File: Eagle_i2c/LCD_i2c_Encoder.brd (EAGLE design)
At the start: 100 x 99 mm, 8 parts, among them J1 455-1750-1-ND, U1 ARDUINOR3-BPLACE

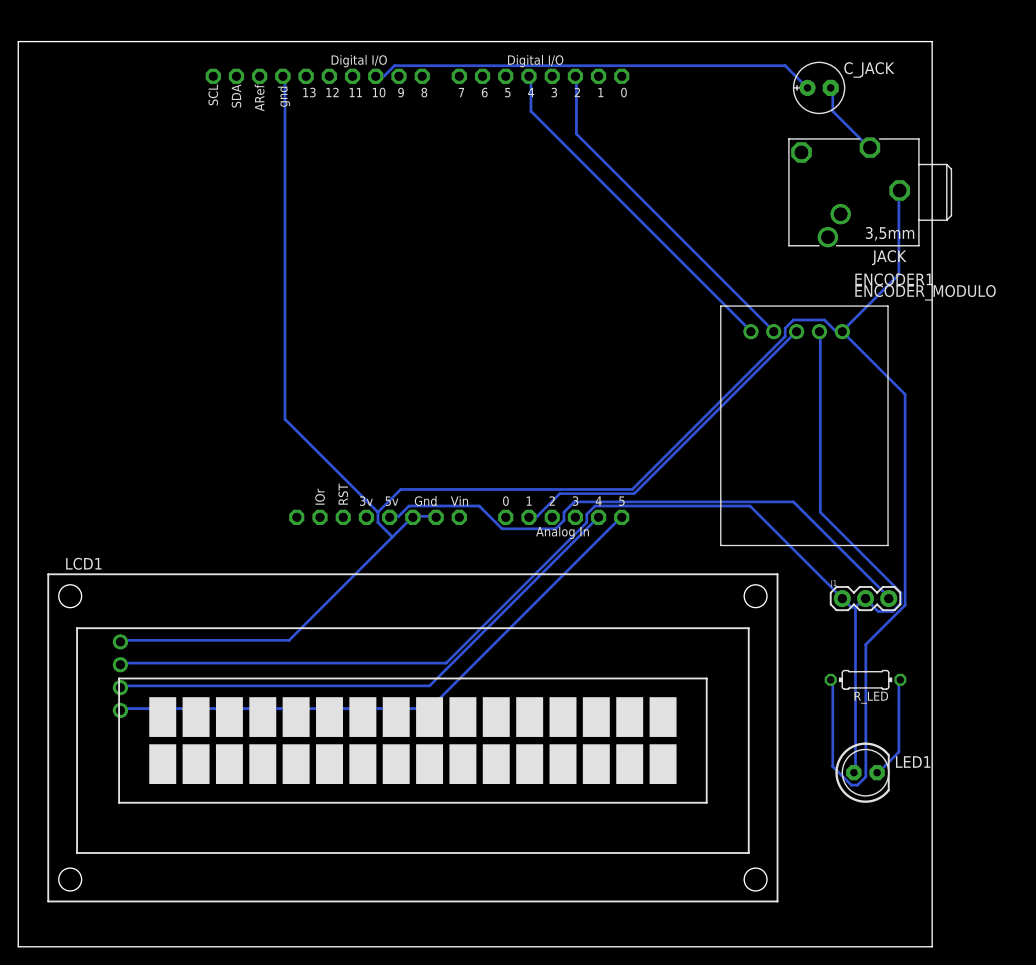
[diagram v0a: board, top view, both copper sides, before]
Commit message: Version final circuito Chladni
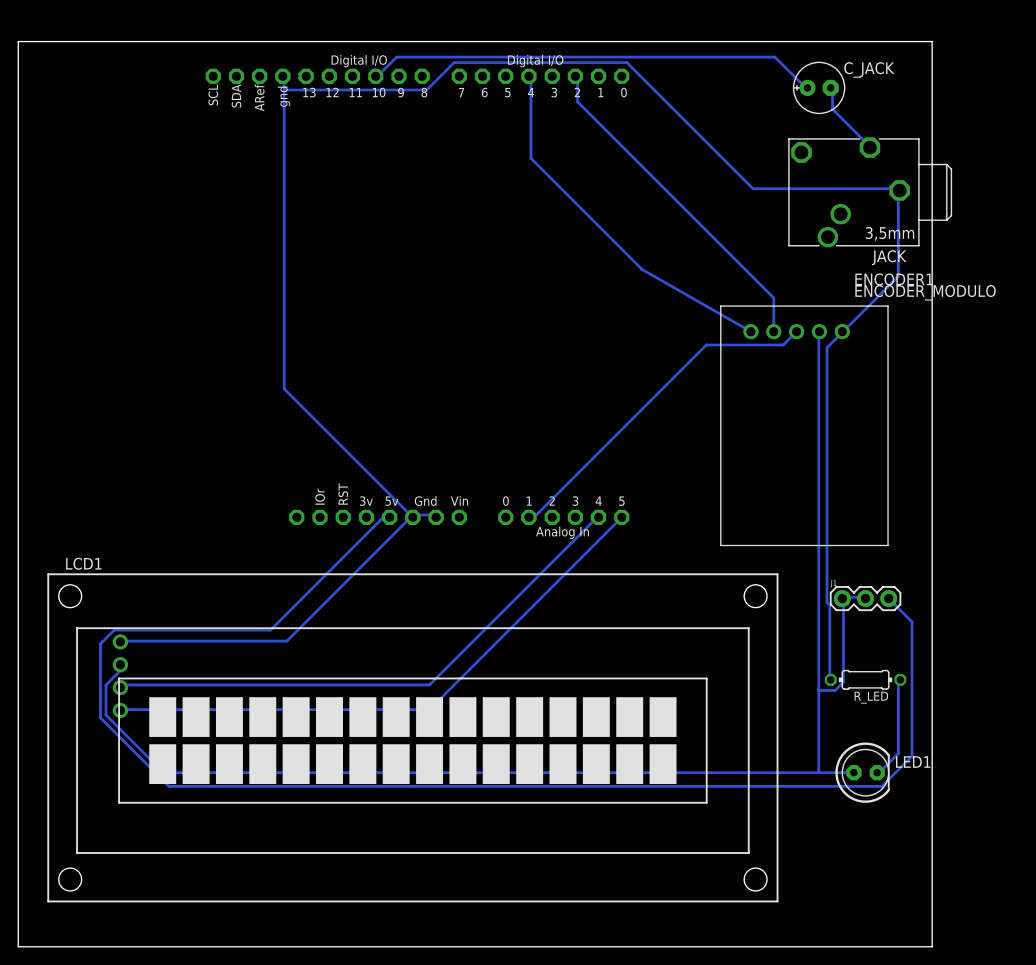
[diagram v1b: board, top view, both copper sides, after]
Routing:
- net N$5: track 62.4 -> 157.0 mm
- net GND: track 242.1 -> 226.3 mm
- net VCC: track 150.8 -> 153.9 mm
- net N$17: track 38.0 -> 40.1 mm
- net N$1: track 48.7 -> 49.5 mm

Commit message: Version para imprimir ICAT, Gerbers incluidos
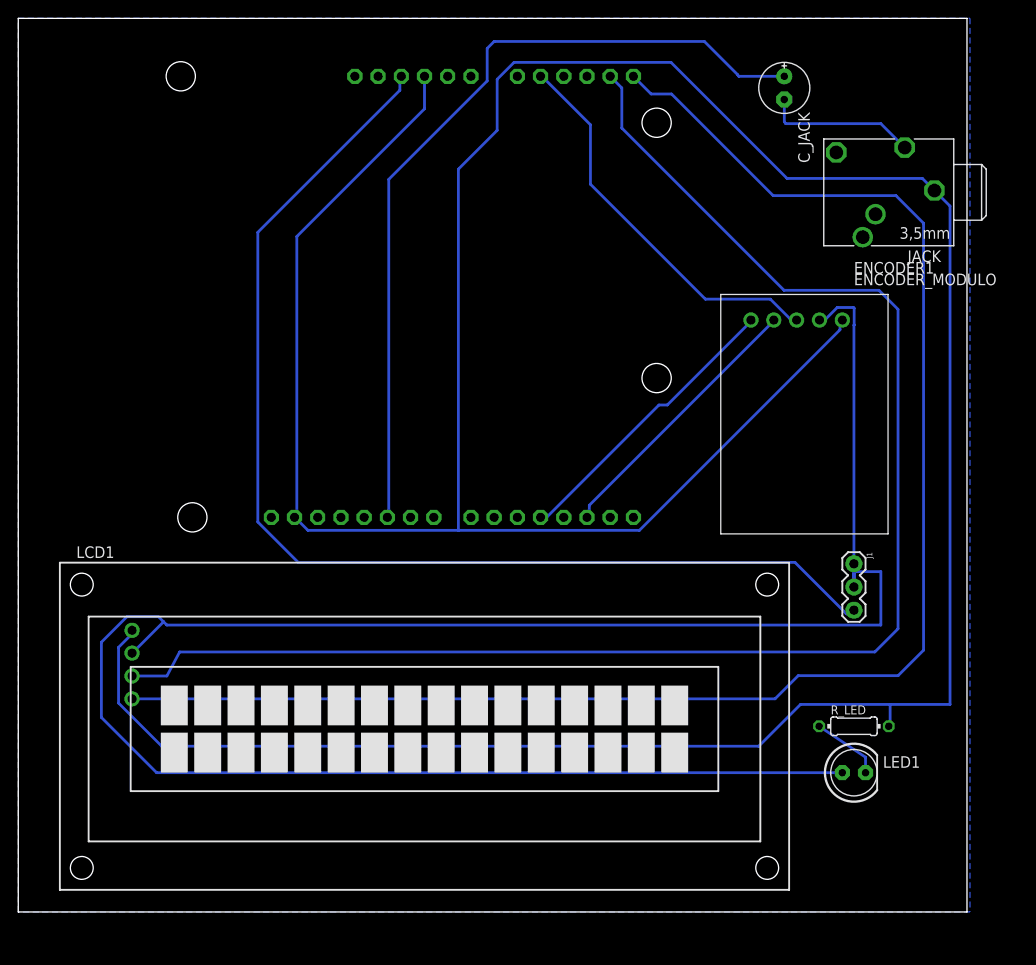
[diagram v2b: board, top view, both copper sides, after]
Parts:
- removed U1: ARDUINOR3-BPLACE, adafruit:ARDUINOR3-BPLACE
- added U$1: ARDUINOUNO, Arduino_Espejo:ARDUINO
- moved R_LED 5.24 mm to (91.4, 5.08), turned to 0 degrees
- moved J1 4.02 mm to (91.4, 22.9), turned to 270 degrees
- moved C_JACK 3.81 mm to (83.8, 74.9), turned to 270 degrees
- moved JACK 3.81 mm to (95.2, 63.5)
- moved LCD1 1.80 mm to (44.5, 5.08)
- moved ENCODER1 1.27 mm to (90.2, 49.5)
- moved LED1 1.27 mm to (91.4, 0.00)
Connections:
- new net GND1: U$1.GND1
- net 3V: now also U$1.3V; no longer U1.3V
- net GND: now also U$1.GND, U$1.GND2; no longer U1.GND, U1.GND1, U1.GND2
- net N$1: now also U$1.D10; no longer U1.D10
- net N$17: now also U$1.D4; no longer U1.D4
- net N$18: now also U$1.D2; no longer U1.D2
- net N$3: now also U$1.A1; no longer U1.A1
- net N$5: now also U$1.5V; no longer U1.5V
- net N$8: now also U$1.A4; no longer U1.A4
- net N$9: now also U$1.A5; no longer U1.A5
- net VIN: now also U$1.VIN; no longer U1.VIN
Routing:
- net GND: track 226.3 -> 393.2 mm
- net N$9: track 63.6 -> 173.9 mm
- net N$8: track 60.0 -> 166.0 mm
- net VCC: track 153.9 -> 234.6 mm
- net N$1: track 49.5 -> 90.3 mm
- net N$5: track 157.0 -> 124.9 mm
- net N$7: track 8.27 -> 16.8 mm
- net N$17: track 40.1 -> 32.0 mm
- net N$18: track 37.1 -> 30.1 mm
- net N$3: track 37.7 -> 42.9 mm
- net N$4: track 11.3 -> 7.80 mm
- added copper zone on layer 16, net GND
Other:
- board size 100 x 99 mm -> 103.8 x 97.8 mm
